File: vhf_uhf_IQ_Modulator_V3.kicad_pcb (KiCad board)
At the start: 2 copper layers, 71 parts, among them J1 CONN_01X03, J2 TEST_1P, J3 Audio-Jack-3, J4 CONN_01X04, J5 SMA Edge FM, Q1 BC817-40, Q2 BC817-40, Q3 BC817-40, U1 TRF3701, U2 MMZ09332BT1, U3 Si570, U4 Orange Pi zero, U5 MCP3421A0T-E/CH

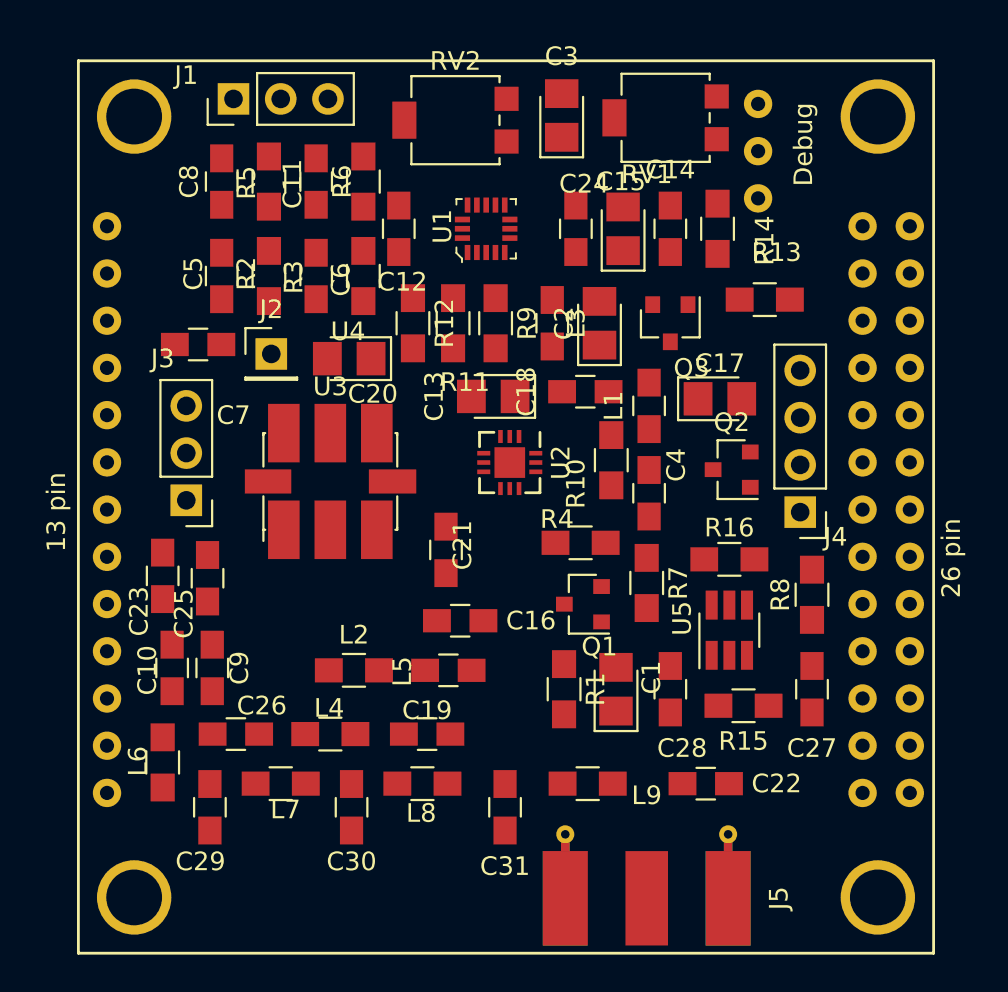
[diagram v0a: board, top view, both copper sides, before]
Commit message: fix resistor
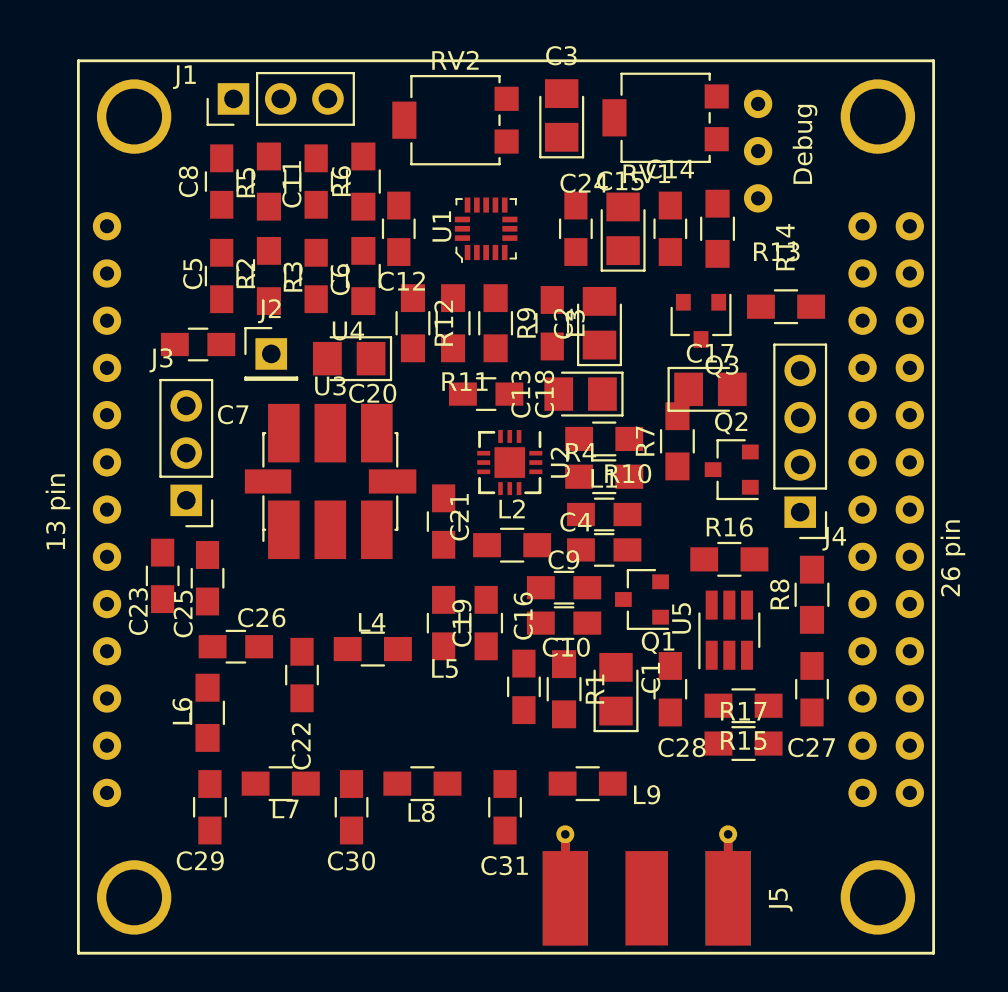
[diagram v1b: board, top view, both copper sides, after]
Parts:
- added R17: 4k7, Resistors_SMD:R_0805_HandSoldering, F.Cu at (184.3, 93.7)
- moved C22 22.5 mm to (160.5, 90.0), turned to 90 degrees
- moved C10 21.2 mm to (174.6, 87.2), turned to 0 degrees
- moved C9 19.4 mm to (174.6, 85.3), turned to 180 degrees
- moved L2 10.8 mm to (171.8, 83.1)
- moved R7 7.80 mm to (180.7, 77.5), turned to 90 degrees
- moved C19 6.76 mm to (170.4, 87.2), turned to 90 degrees
- moved L1 6.32 mm to (176.8, 81.4), turned to 180 degrees
- moved C18 5.34 mm to (170.4, 74.9), turned to 0 degrees
- moved L4 5.11 mm to (164.3, 88.6)
- moved C16 4.94 mm to (172.5, 90.7), turned to 270 degrees
- moved C13 4.70 mm to (175.5, 74.9)
- moved C26 4.70 mm to (157.0, 88.5)
- moved C4 3.89 mm to (176.8, 83.3), turned to 180 degrees
- moved R4 3.78 mm to (176.8, 79.4)
- moved L6 3.60 mm to (155.4, 92.1)
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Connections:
- Q1 pad 1: PA01 -> Net-(Q1-Pad1)
- U2 pad 4: (no net) -> Net-(U2-Pad4)
